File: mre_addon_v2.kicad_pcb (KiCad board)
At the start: 2 copper layers, 80.6 x 48.4 mm, 86 parts, among them J1 TC2030, J10 Molex_Micro-Fit_3.0_43045-080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, J10 Molex_Micro-Fit_3.0_43045-081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, J15 microSD_HC_Wuerth_693072010801, J15x MICRO-SDCARD-CONNECTOR-330006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, J2 Conn_01x06_Male, J20 Conn_02x05_Odd_Even-Connector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, J21 Soldering PAD for 12V_MREL, J3 Conn_01x03_Male, J30 Conn_02x05_Odd_Even-Connector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, J40 CONN_Molex, J40x Molex_Micro-Fit_3.0_43045-021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, J41 CONN_Sparkfun, Q1 BTS3028, SW1 SW_Push, U0 wideband_MRE_R055, U1 STM32F072CBUx, U2 MCP6004, U3 AD8628, U3 SO-8_3.9x4.9mm_P1.27mm, U4 REF3033, U5 TJA1051T-3, U6 MAX31855KASA

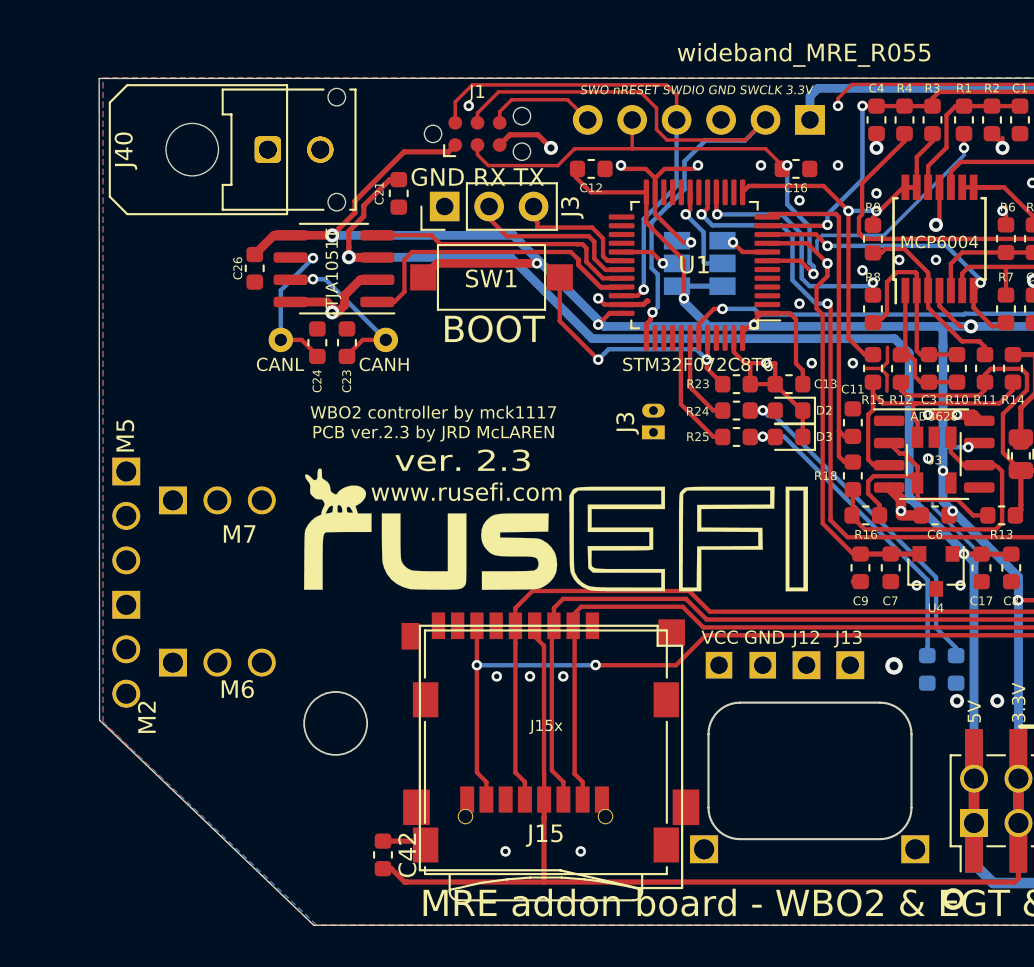
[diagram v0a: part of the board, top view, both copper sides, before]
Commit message: Add files via upload
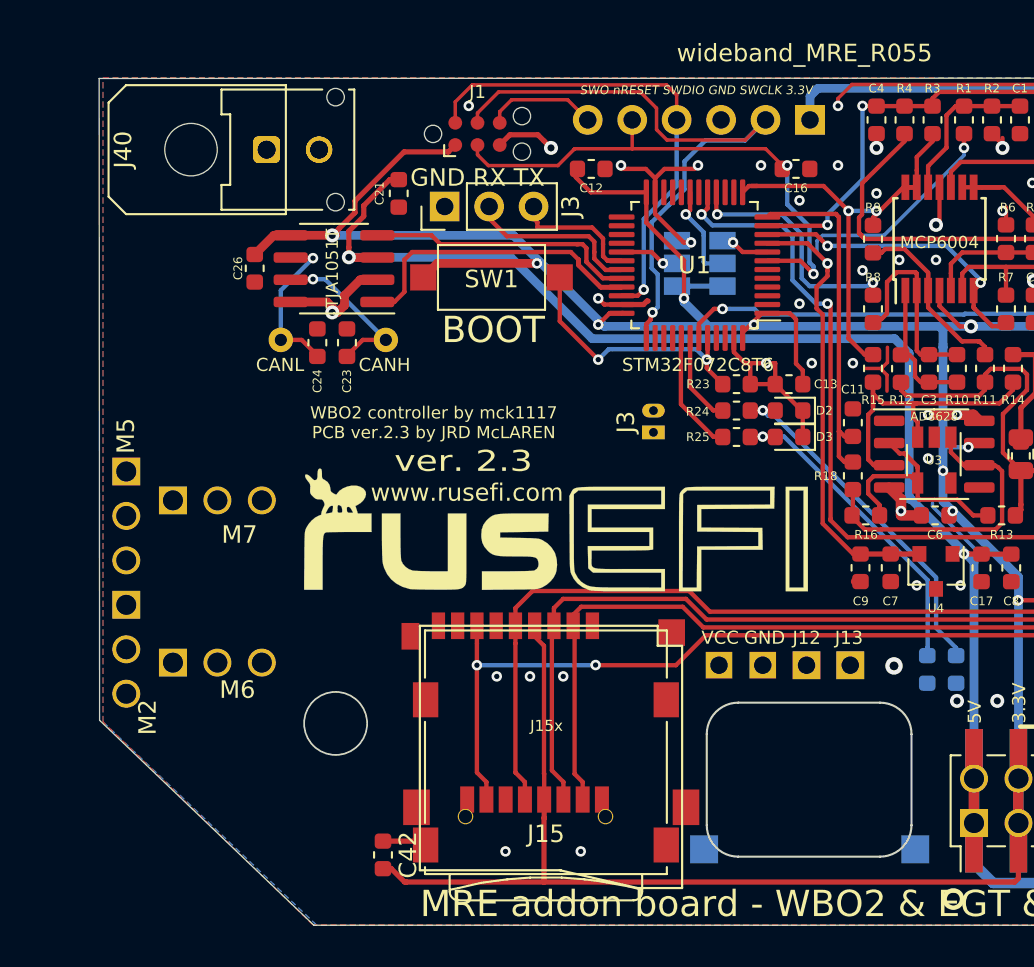
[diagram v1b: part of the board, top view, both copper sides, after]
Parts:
- moved J40 0.07 mm to (84.5, 129.9)
- moved J40x 0.07 mm to (84.5, 129.9)
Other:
- outline, holes or cut-outs redrawn
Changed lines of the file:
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@@
     (mod_text_width 0.15)
     (pad_size 1.6 1.6)
-    (pad_drill 0.8)
+    (pad_drill 0)
     (pad_to_mask_clearance 0.051)
     (solder_mask_min_width 0.25)
@@
   )
   (module Connector_Molex:Molex_Micro-Fit_3.0_43045-0212_2x01_P3.00mm_Vertical (layer F.Cu)
-    (at 84.62 129.9 90)
+    (at 84.55 129.9 90)
     (descr "Molex Micro-Fit 3.0 Connector System, 43045-0212 (compatible alternatives: 43045-0213, 43045-0224), 1 Pins per row (http://www.molex.com/pdm_docs/sd/430450212_sd.pdf), generated with kicad-footprint-generator")
     (tags "connector Molex Micro-Fit_3.0 side entry")
@@
   )
   (module Connector_Molex:Molex_Micro-Fit_3.0_43045-0200_2x01_P3.00mm_Horizontal (layer F.Cu)
-    (at 84.62 129.9 90)
+    (at 84.55 129.9 90)
     (descr "Molex Micro-Fit 3.0 Connector System, 43045-0200 (alternative finishes: 43045-020x), 1 Pins per row (https://www.molex.com/pdm_docs/sd/430450201_sd.pdf), generated with kicad-footprint-generator")
     (tags "connector Molex Micro-Fit_3.0 horizontal")
@@
     (pad M12 thru_hole circle (at -38.7096 -9.6824 270) (size 1.6 1.6) (drill 1.15) (layers *.Cu *.Mask))
     (pad M13 thru_hole circle (at -38.7096 -12.2224 270) (size 1.6 1.6) (drill 1.15) (layers *.Cu *.Mask))
-    (pad M3 thru_hole rect (at -6.3246 -21.1124 270) (size 1.6 1.6) (drill 1.15) (layers *.Cu *.Mask))
-    (pad M4 thru_hole rect (at 5.7404 -21.1124 270) (size 1.6 1.6) (drill 1.15) (layers *.Cu *.Mask))
+    (pad "" connect rect (at -6.3246 -21.1124 270) (size 1.6 1.6) (layers B.Cu B.Mask))
+    (pad "" connect rect (at 5.7404 -21.1124 270) (size 1.6 1.6) (layers B.Cu B.Mask))
     (pad M21 thru_hole rect (at 38.7604 -7.1424 270) (size 1.6 1.6) (drill 1.15) (layers *.Cu *.Mask))
     (pad M22 thru_hole circle (at 38.7604 -9.6824 270) (size 1.6 1.6) (drill 1.15) (layers *.Cu *.Mask))
@@
   (gr_circle (center 98.4 147.05) (end 103.4 147.05) (layer B.SilkS) (width 0.12))
   (gr_circle (center 96.95 145) (end 101.95 145) (layer B.SilkS) (width 0.12))
-  (gr_line (start 111.6 169.3) (end 119.6 169.3) (layer Edge.Cuts) (width 0.12))
-  (gr_line (start 121.4 167.5) (end 121.4 163.3) (layer Edge.Cuts) (width 0.12))
-  (gr_line (start 109.8 163.3) (end 109.8 167.5) (layer Edge.Cuts) (width 0.12))
-  (gr_line (start 111.6 161.5) (end 119.6 161.5) (layer Edge.Cuts) (width 0.12))
-  (gr_arc (start 111.6 163.3) (end 111.6 161.5) (angle -90) (layer Edge.Cuts) (width 0.12))
+  (gr_line (start 111.5 170.3) (end 119.6 170.3) (layer Edge.Cuts) (width 0.12))
+  (gr_line (start 121.4 168.5) (end 121.4 163.3) (layer Edge.Cuts) (width 0.12))
+  (gr_line (start 109.7 163.3) (end 109.7 168.5) (layer Edge.Cuts) (width 0.12))
+  (gr_line (start 111.5 161.5) (end 119.6 161.5) (layer Edge.Cuts) (width 0.12))
+  (gr_arc (start 111.5 163.3) (end 111.5 161.5) (angle -90) (layer Edge.Cuts) (width 0.12))
   (gr_arc (start 119.6 163.3) (end 121.4 163.3) (angle -90) (layer Edge.Cuts) (width 0.12))
-  (gr_arc (start 111.6 167.5) (end 109.8 167.5) (angle -90) (layer Edge.Cuts) (width 0.12))
-  (gr_arc (start 119.6 167.5) (end 119.6 169.3) (angle -90) (layer Edge.Cuts) (width 0.12))
+  (gr_arc (start 111.5 168.5) (end 109.7 168.5) (angle -90) (layer Edge.Cuts) (width 0.12))
+  (gr_arc (start 119.6 168.5) (end 119.6 170.3) (angle -90) (layer Edge.Cuts) (width 0.12))
   (gr_line (start 98.4 147.6) (end 98.4 146.5) (layer B.SilkS) (width 0.12))
   (gr_line (start 97.85 147.05) (end 98.95 147.05) (layer B.SilkS) (width 0.12))
